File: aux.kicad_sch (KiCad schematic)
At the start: 14 parts, among them J401 FREE, J402 AUX0, J403 AUX1, J404 AUX2, J405 AUX0OUT, J406 AUX1OUT, J407 AUX2OUT, J408 AUX3, J409 AUX3OUT, J410 UARTBUSV, J411 CANBUSV, J412 I2C, J413 CAN, J414 UART

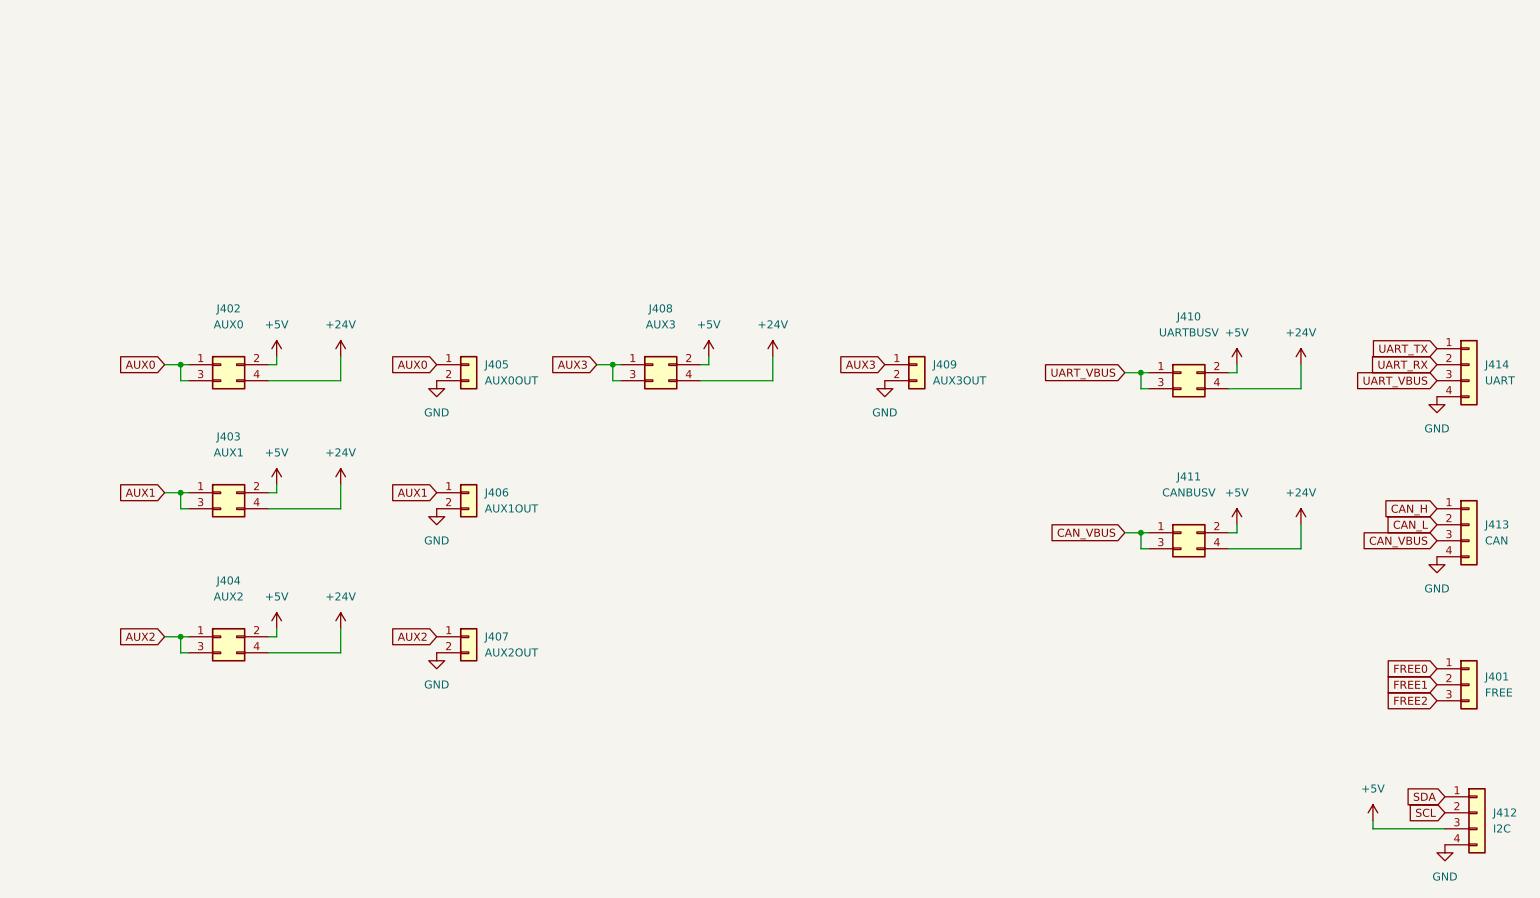
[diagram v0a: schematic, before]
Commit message: update board
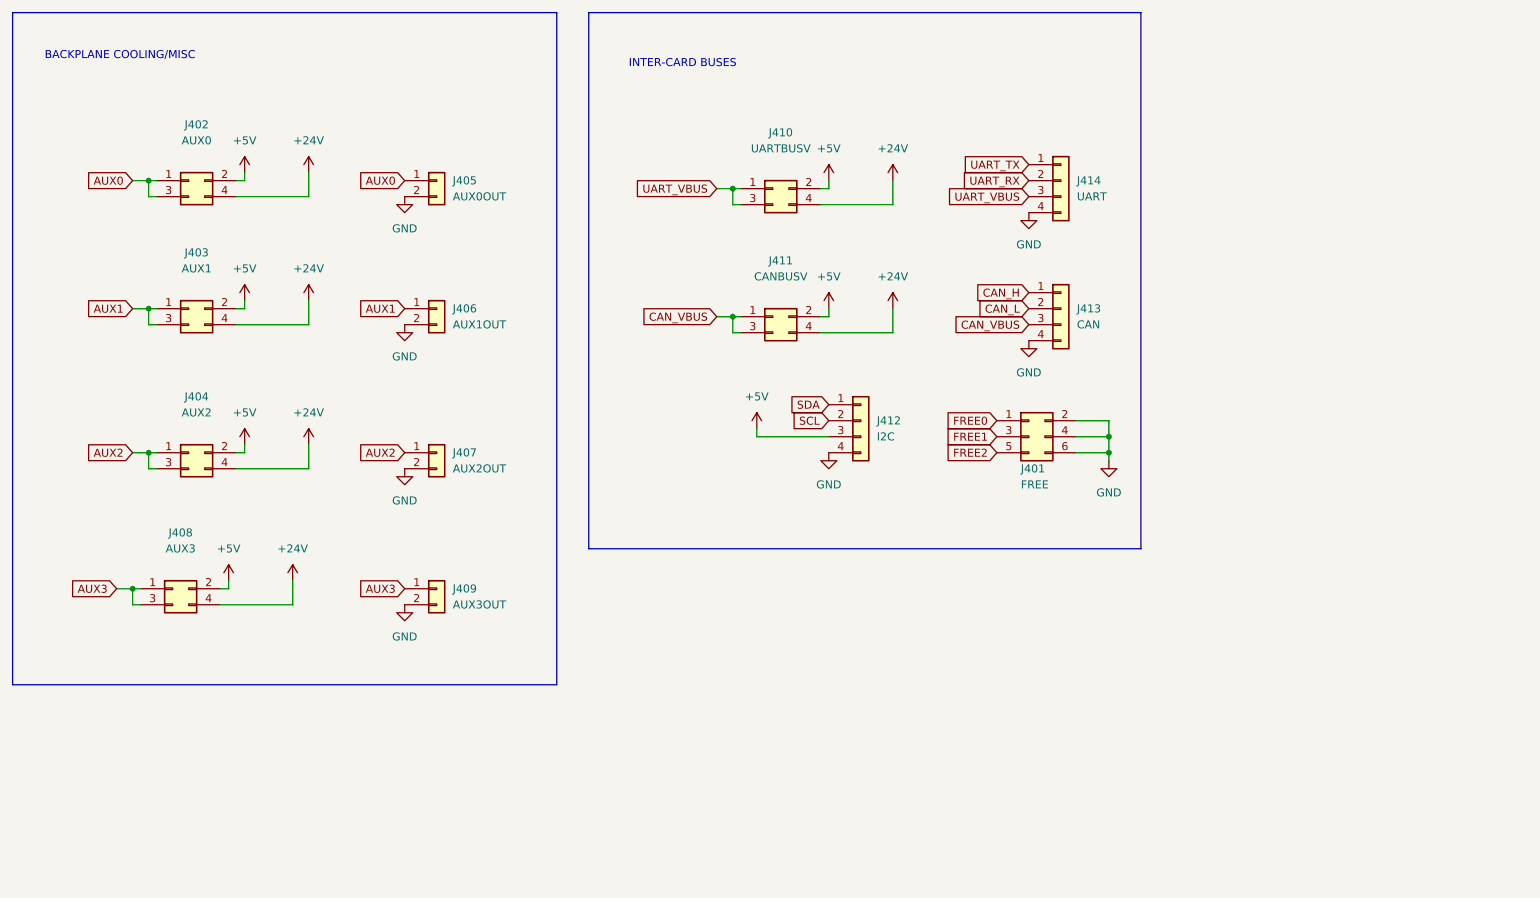
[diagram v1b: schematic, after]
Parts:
- J401: footprint Connector_PinHeader_2.54mm:PinHeader_1x03_P2.54mm_Vertical -> Connector_PinHeader_2.54mm:PinHeader_2x03_P2.54mm_Vertical; symbol Connector_Generic:Conn_01x03 -> Connector_Generic:Conn_02x03_Odd_Even
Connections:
- net FREE1: now also J401.3 (Pin_3); no longer J401.2 (Pin_2)
- net FREE2: now also J401.5 (Pin_5); no longer J401.3 (Pin_3)
- net GND: now also J401.2 (Pin_2), J401.4 (Pin_4), J401.6 (Pin_6)
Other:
- note added: "BACKPLANE COOLING/MISC"
- note added: "INTER-CARD BUSES"
- moved on the sheet: J402, J403, J404, J405, J406, J407, J408, J409, J410, J411, J412, J413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
